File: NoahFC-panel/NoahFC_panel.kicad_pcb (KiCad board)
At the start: 2 copper layers, 97 x 97 mm, 112 parts, among them J1 CH1, J10 GND, J11 CH1, J12 CH2, J13 MPU6050, J14 FTDI, J15 8.4V, J16 CH3, J17 PPM, J18 GPS, J19 CH4, J2 CH2, J20 GND, J21 CH1, J22 CH2, J23 MPU6050, J24 FTDI, J25 8.4V, J26 CH3, J27 PPM, J28 GPS, J29 CH4, J3 MPU6050, J30 GND, J31 CH1, J32 CH2, J33 MPU6050, J34 FTDI, J35 8.4V, J36 CH3, J37 PPM, J38 GPS, J39 CH4, J4 FTDI, J40 GND, J5 8.4V, J6 CH3, J7 PPM, J8 GPS, J9 CH4, U1 ATmega328-A, U2 ATmega328-A, U3 AMS1117-5.0, U4 AMS1117-5.0, U5 ATmega328-A, U6 AMS1117-5.0, U7 ATmega328-A, U8 AMS1117-5.0, Y1 16Mhz, Y2 16Mhz, Y3 16Mhz, Y4 16Mhz

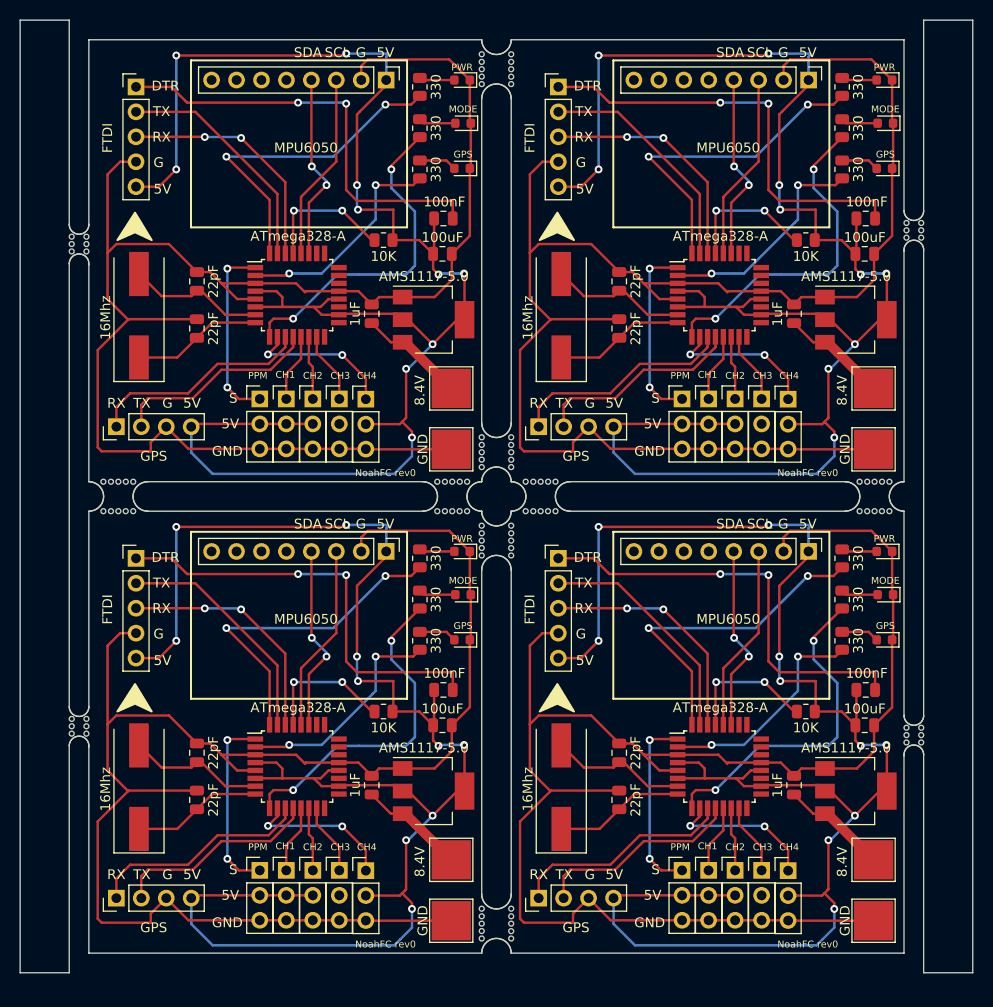
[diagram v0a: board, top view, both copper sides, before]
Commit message: fill board
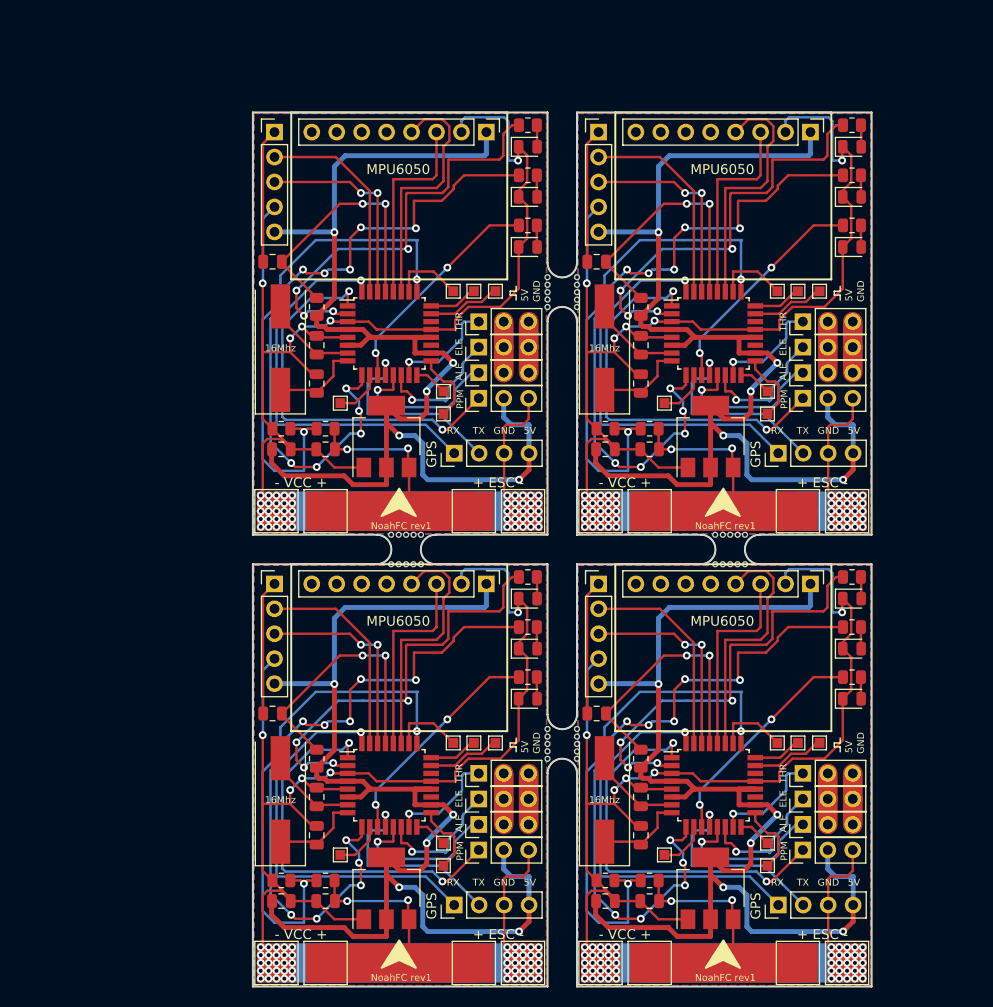
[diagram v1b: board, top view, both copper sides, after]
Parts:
- removed the C1 at (96.9, 72.9)
- removed C10, C15, C20: 100uF, Capacitor_SMD:C_0805_2012Metric
- removed C11, C12, C16, C17, C6, C7: 22pF, Capacitor_SMD:C_0805_2012Metric
- removed C13, C18, C8: 100nF, Capacitor_SMD:C_0805_2012Metric
- removed C14, C19, C9: 1uF, Capacitor_SMD:C_0805_2012Metric
- removed the C2 at (96.9, 77.7)
- removed the C3 at (122.0, 66.5)
- removed the C4 at (114.7, 76.2)
- removed the C5 at (121.9, 70.1)
- removed the D1 at (123.9, 52.4)
- removed D10, D4, D7: PWR, LED_SMD:LED_0603_1608Metric
- removed D11, D5, D8: GPS, LED_SMD:LED_0603_1608Metric
- removed D12, D6, D9: MODE, LED_SMD:LED_0603_1608Metric
- removed the D2 at (123.9, 61.4)
- removed the D3 at (124.0, 56.8)
- removed the J1 at (106.0, 84.9)
- removed the J10 at (122.8, 90.0)
- removed the J11 at (149.0, 84.9)
- removed the J12 at (151.7, 84.9)
- removed the J13 at (159.2, 52.4)
- removed the J14 at (133.7, 53.1)
- removed the J15 at (165.8, 83.8)
- removed the J16 at (154.4, 84.9)
- removed the J17 at (146.3, 84.9)
- removed J18, J28, J38: GPS, Connector_PinHeader_2.54mm:PinHeader_1x04_P2.54mm_Vertical
- removed J19, J29, J39: CH4, Connector_PinHeader_2.54mm:PinHeader_1x03_P2.54mm_Vertical
- removed the J2 at (108.7, 84.9)
- removed J20, J30, J40: GND, TestPoint:TestPoint_Pad_4.0x4.0mm
- removed J21, J31: CH1, Connector_PinHeader_2.54mm:PinHeader_1x03_P2.54mm_Vertical
- removed J22, J32: CH2, Connector_PinHeader_2.54mm:PinHeader_1x03_P2.54mm_Vertical
- removed J23, J33: MPU6050, Connector_PinHeader_2.54mm:PinHeader_1x08_P2.54mm_Vertical
- removed J24, J34: FTDI, Connector_PinHeader_2.54mm:PinHeader_1x05_P2.54mm_Vertical
- removed J25, J35: 8.4V, TestPoint:TestPoint_Pad_4.0x4.0mm
- removed J26, J36: CH3, Connector_PinHeader_2.54mm:PinHeader_1x03_P2.54mm_Vertical
- removed J27, J37: PPM, Connector_PinHeader_2.54mm:PinHeader_1x03_P2.54mm_Vertical
- removed the J3 at (116.2, 52.4)
- removed the J4 at (90.7, 53.1)
- removed the J5 at (122.8, 83.8)
- removed the J6 at (111.4, 84.9)
- removed the J7 at (103.3, 84.9)
- removed the J8 at (88.7, 87.7)
- removed the J9 at (114.1, 84.9)
- removed the R1 at (115.9, 68.7)
- removed R10, R11, R12, R14, R15, R16, R7, R8: 330, Resistor_SMD:R_0805_2012Metric
- removed R13, R9: 10K, Resistor_SMD:R_0805_2012Metric
- removed the R2 at (119.6, 53.1)
- removed the R3 at (119.6, 61.5)
- removed the R4 at (119.6, 57.3)
- removed the R5 at (158.9, 68.7)
- removed the R6 at (162.6, 53.1)
- removed the U1 at (107.1, 74.3)
- removed U2, U5, U7: ATmega328-A, Package_QFP:TQFP-32_7x7mm_P0.8mm
- removed the U3 at (121.0, 76.8)
- removed U4, U6, U8: AMS1117-5.0, Package_TO_SOT_SMD:SOT-223-3_TabPin2
- removed the Y1 at (91.0, 76.4)
- removed Y2, Y3, Y4: 16Mhz, Crystal:Crystal_SMD_HC49-SD
- removed the mouse-bite-3mm-slot at (84.9, 118.2)
- removed the mouse-bite-3mm-slot at (84.9, 69.1)
- removed the mouse-bite-3mm-slot at (131.9, 94.8)
- removed the mouse-bite-3mm-slot at (88.9, 94.8)
- removed the mouse-bite-3mm-slot at (169.9, 67.7)
- removed the mouse-bite-3mm-slot at (127.4, 51.3)
- removed the mouse-bite-3mm-slot at (127.4, 99.3)
- removed the mouse-bite-3mm-slot at (127.4, 90.3)
- removed the mouse-bite-3mm-slot at (127.4, 138.3)
- removed the mouse-bite-3mm-slot at (122.9, 94.8)
- removed the mouse-bite-3mm-slot at (169.9, 119.1)
- removed the mouse-bite-3mm-slot at (165.9, 94.8)
- added C1: 22pF, Capacitor_SMD:C_0805_2012Metric, F.Cu at (142.1, 125.4)
- added C1: 22pF, Capacitor_SMD:C_0805_2012Metric, F.Cu at (142.1, 79.4)
- added C1: 22pF, Capacitor_SMD:C_0805_2012Metric, F.Cu at (109.1, 125.4)
- added C1: 22pF, Capacitor_SMD:C_0805_2012Metric, F.Cu at (109.1, 79.4)
- added C2: 22pF, Capacitor_SMD:C_0805_2012Metric, F.Cu at (142.1, 129.3)
- added C2: 22pF, Capacitor_SMD:C_0805_2012Metric, F.Cu at (142.1, 83.3)
- added C2: 22pF, Capacitor_SMD:C_0805_2012Metric, F.Cu at (109.1, 83.3)
- added C2: 22pF, Capacitor_SMD:C_0805_2012Metric, F.Cu at (109.1, 129.3)
- added C3: 1nF, Capacitor_SMD:C_0805_2012Metric, F.Cu at (137.6, 70.9)
- added C3: 1nF, Capacitor_SMD:C_0805_2012Metric, F.Cu at (104.6, 70.9)
- added C3: 1nF, Capacitor_SMD:C_0805_2012Metric, F.Cu at (104.6, 116.9)
- added C3: 1nF, Capacitor_SMD:C_0805_2012Metric, F.Cu at (137.6, 116.9)
- added C4: 1uF, Capacitor_SMD:C_0805_2012Metric, F.Cu at (110.0, 136.0)
- added C4: 1uF, Capacitor_SMD:C_0805_2012Metric, F.Cu at (110.0, 90.0)
- added C4: 1uF, Capacitor_SMD:C_0805_2012Metric, F.Cu at (143.0, 90.0)
- added C4: 1uF, Capacitor_SMD:C_0805_2012Metric, F.Cu at (143.0, 136.0)
- added C5: 10uF, Capacitor_SMD:C_0805_2012Metric, F.Cu at (105.5, 136.0)
- added C5: 10uF, Capacitor_SMD:C_0805_2012Metric, F.Cu at (105.5, 90.0)
- added C5: 10uF, Capacitor_SMD:C_0805_2012Metric, F.Cu at (138.5, 90.0)
- added C5: 10uF, Capacitor_SMD:C_0805_2012Metric, F.Cu at (138.5, 136.0)
- added D1: GPS, LED_SMD:LED_0805_2012Metric, F.Cu at (130.6, 110.3)
- added D1: GPS, LED_SMD:LED_0805_2012Metric, F.Cu at (163.6, 110.3)
- added D1: GPS, LED_SMD:LED_0805_2012Metric, F.Cu at (130.6, 64.3)
- added D1: GPS, LED_SMD:LED_0805_2012Metric, F.Cu at (163.6, 64.3)
- added D2: MODE, LED_SMD:LED_0805_2012Metric, F.Cu at (130.6, 59.2)
- added D2: MODE, LED_SMD:LED_0805_2012Metric, F.Cu at (163.6, 59.2)
- added D2: MODE, LED_SMD:LED_0805_2012Metric, F.Cu at (163.6, 105.2)
- added D2: MODE, LED_SMD:LED_0805_2012Metric, F.Cu at (130.6, 105.2)
- added D3: PWR, LED_SMD:LED_0805_2012Metric, F.Cu at (163.6, 69.4)
- added D3: PWR, LED_SMD:LED_0805_2012Metric, F.Cu at (163.6, 115.4)
- added D3: PWR, LED_SMD:LED_0805_2012Metric, F.Cu at (130.6, 115.4)
- added D3: PWR, LED_SMD:LED_0805_2012Metric, F.Cu at (130.6, 69.4)
- added J1: ALE, Connector_PinHeader_2.54mm:PinHeader_1x03_P2.54mm_Vertical, F.Cu at (125.6, 128.2)
- added J1: ALE, Connector_PinHeader_2.54mm:PinHeader_1x03_P2.54mm_Vertical, F.Cu at (158.6, 128.2)
- added J1: ALE, Connector_PinHeader_2.54mm:PinHeader_1x03_P2.54mm_Vertical, F.Cu at (158.6, 82.2)
- added J1: ALE, Connector_PinHeader_2.54mm:PinHeader_1x03_P2.54mm_Vertical, F.Cu at (125.6, 82.2)
- added J10: GND, TestPoint:TestPoint_Pad_4.0x4.0mm, F.Cu at (105.0, 142.3)
- added J10: GND, TestPoint:TestPoint_Pad_4.0x4.0mm, F.Cu at (138.0, 142.3)
- added J10: GND, TestPoint:TestPoint_Pad_4.0x4.0mm, F.Cu at (138.0, 96.3)
- added J10: GND, TestPoint:TestPoint_Pad_4.0x4.0mm, F.Cu at (105.0, 96.3)
- added J11: SCK, TestPoint:TestPoint_Pad_1.0x1.0mm, F.Cu at (155.0, 132.4)
- added J11: SCK, TestPoint:TestPoint_Pad_1.0x1.0mm, F.Cu at (155.0, 86.4)
- added J11: SCK, TestPoint:TestPoint_Pad_1.0x1.0mm, F.Cu at (122.0, 132.4)
- added J11: SCK, TestPoint:TestPoint_Pad_1.0x1.0mm, F.Cu at (122.0, 86.4)
- added J12: MISO, TestPoint:TestPoint_Pad_1.0x1.0mm, F.Cu at (155.0, 130.1)
- added J12: MISO, TestPoint:TestPoint_Pad_1.0x1.0mm, F.Cu at (155.0, 84.1)
- added J12: MISO, TestPoint:TestPoint_Pad_1.0x1.0mm, F.Cu at (122.0, 130.1)
- added J12: MISO, TestPoint:TestPoint_Pad_1.0x1.0mm, F.Cu at (122.0, 84.1)
- added J13: VCC, TestPoint:TestPoint_Pad_4.0x4.0mm, F.Cu at (158.1, 142.3)
- added J13: VCC, TestPoint:TestPoint_Pad_4.0x4.0mm, F.Cu at (158.1, 96.3)
- added J13: VCC, TestPoint:TestPoint_Pad_4.0x4.0mm, F.Cu at (125.1, 142.3)
- added J13: VCC, TestPoint:TestPoint_Pad_4.0x4.0mm, F.Cu at (125.1, 96.3)
- added J14: GND, TestPoint:TestPoint_Pad_4.0x4.0mm, F.Cu at (130.1, 142.3)
- added J14: GND, TestPoint:TestPoint_Pad_4.0x4.0mm, F.Cu at (163.1, 142.3)
- added J14: GND, TestPoint:TestPoint_Pad_4.0x4.0mm, F.Cu at (130.1, 96.3)
- added J14: GND, TestPoint:TestPoint_Pad_4.0x4.0mm, F.Cu at (163.1, 96.3)
- added J15: A1, TestPoint:TestPoint_Pad_1.0x1.0mm, F.Cu at (125.1, 73.9)
- added J15: A1, TestPoint:TestPoint_Pad_1.0x1.0mm, F.Cu at (158.1, 119.9)
- added J15: A1, TestPoint:TestPoint_Pad_1.0x1.0mm, F.Cu at (125.1, 119.9)
- added J15: A1, TestPoint:TestPoint_Pad_1.0x1.0mm, F.Cu at (158.1, 73.9)
- added J16: A3, TestPoint:TestPoint_Pad_1.0x1.0mm, F.Cu at (156.0, 73.9)
- added J16: A3, TestPoint:TestPoint_Pad_1.0x1.0mm, F.Cu at (123.0, 119.9)
- added J16: A3, TestPoint:TestPoint_Pad_1.0x1.0mm, F.Cu at (156.0, 119.9)
- added J16: A3, TestPoint:TestPoint_Pad_1.0x1.0mm, F.Cu at (123.0, 73.9)
- added J17: D6, TestPoint:TestPoint_Pad_1.0x1.0mm, F.Cu at (111.5, 85.3)
- added J17: D6, TestPoint:TestPoint_Pad_1.0x1.0mm, F.Cu at (144.5, 131.3)
- added J17: D6, TestPoint:TestPoint_Pad_1.0x1.0mm, F.Cu at (144.5, 85.3)
- added J17: D6, TestPoint:TestPoint_Pad_1.0x1.0mm, F.Cu at (111.5, 131.3)
- added J2: ELE, Connector_PinHeader_2.54mm:PinHeader_1x03_P2.54mm_Vertical, F.Cu at (125.6, 79.6)
- added J2: ELE, Connector_PinHeader_2.54mm:PinHeader_1x03_P2.54mm_Vertical, F.Cu at (158.6, 79.6)
- added J2: ELE, Connector_PinHeader_2.54mm:PinHeader_1x03_P2.54mm_Vertical, F.Cu at (158.6, 125.6)
- added J2: ELE, Connector_PinHeader_2.54mm:PinHeader_1x03_P2.54mm_Vertical, F.Cu at (125.6, 125.6)
- added J3: MPU6050, Connector_PinHeader_2.54mm:PinHeader_1x08_P2.54mm_Vertical, F.Cu at (126.4, 103.7)
- added J3: MPU6050, Connector_PinHeader_2.54mm:PinHeader_1x08_P2.54mm_Vertical, F.Cu at (126.4, 57.7)
- added J3: MPU6050, Connector_PinHeader_2.54mm:PinHeader_1x08_P2.54mm_Vertical, F.Cu at (159.4, 57.7)
- added J3: MPU6050, Connector_PinHeader_2.54mm:PinHeader_1x08_P2.54mm_Vertical, F.Cu at (159.4, 103.7)
- added J4: FTDI, Connector_PinHeader_2.54mm:PinHeader_1x05_P2.54mm_Vertical, F.Cu at (137.8, 103.7)
- added J4: FTDI, Connector_PinHeader_2.54mm:PinHeader_1x05_P2.54mm_Vertical, F.Cu at (104.8, 57.7)
- added J4: FTDI, Connector_PinHeader_2.54mm:PinHeader_1x05_P2.54mm_Vertical, F.Cu at (104.8, 103.7)
- added J4: FTDI, Connector_PinHeader_2.54mm:PinHeader_1x05_P2.54mm_Vertical, F.Cu at (137.8, 57.7)
- added J5: VCC, TestPoint:TestPoint_Pad_4.0x4.0mm, F.Cu at (143.0, 96.3)
- added J5: VCC, TestPoint:TestPoint_Pad_4.0x4.0mm, F.Cu at (110.0, 142.3)
- added J5: VCC, TestPoint:TestPoint_Pad_4.0x4.0mm, F.Cu at (143.0, 142.3)
- added J5: VCC, TestPoint:TestPoint_Pad_4.0x4.0mm, F.Cu at (110.0, 96.3)
- added J6: THR, Connector_PinHeader_2.54mm:PinHeader_1x03_P2.54mm_Vertical, F.Cu at (125.6, 77.0)
- added J6: THR, Connector_PinHeader_2.54mm:PinHeader_1x03_P2.54mm_Vertical, F.Cu at (158.6, 77.0)
- added J6: THR, Connector_PinHeader_2.54mm:PinHeader_1x03_P2.54mm_Vertical, F.Cu at (125.6, 123.0)
- added J6: THR, Connector_PinHeader_2.54mm:PinHeader_1x03_P2.54mm_Vertical, F.Cu at (158.6, 123.0)
- added J7: PPM, Connector_PinHeader_2.54mm:PinHeader_1x03_P2.54mm_Vertical, F.Cu at (125.6, 84.8)
- added J7: PPM, Connector_PinHeader_2.54mm:PinHeader_1x03_P2.54mm_Vertical, F.Cu at (158.6, 130.8)
- added J7: PPM, Connector_PinHeader_2.54mm:PinHeader_1x03_P2.54mm_Vertical, F.Cu at (125.6, 130.8)
- added J7: PPM, Connector_PinHeader_2.54mm:PinHeader_1x03_P2.54mm_Vertical, F.Cu at (158.6, 84.8)
- added J8: GPS, Connector_PinHeader_2.54mm:PinHeader_1x04_P2.54mm_Vertical, F.Cu at (156.1, 136.4)
- added J8: GPS, Connector_PinHeader_2.54mm:PinHeader_1x04_P2.54mm_Vertical, F.Cu at (123.1, 136.4)
- added J8: GPS, Connector_PinHeader_2.54mm:PinHeader_1x04_P2.54mm_Vertical, F.Cu at (123.1, 90.4)
- added J8: GPS, Connector_PinHeader_2.54mm:PinHeader_1x04_P2.54mm_Vertical, F.Cu at (156.1, 90.4)
- added J9: A0, TestPoint:TestPoint_Pad_1.0x1.0mm, F.Cu at (160.3, 73.9)
- added J9: A0, TestPoint:TestPoint_Pad_1.0x1.0mm, F.Cu at (127.3, 119.9)
- added J9: A0, TestPoint:TestPoint_Pad_1.0x1.0mm, F.Cu at (127.3, 73.9)
- added J9: A0, TestPoint:TestPoint_Pad_1.0x1.0mm, F.Cu at (160.3, 119.9)
- added R1: 10K, Resistor_SMD:R_0805_2012Metric, F.Cu at (142.1, 75.5)
- added R1: 10K, Resistor_SMD:R_0805_2012Metric, F.Cu at (109.1, 75.5)
- added R1: 10K, Resistor_SMD:R_0805_2012Metric, F.Cu at (109.1, 121.5)
- added R1: 10K, Resistor_SMD:R_0805_2012Metric, F.Cu at (142.1, 121.5)
- added R2: 330, Resistor_SMD:R_0805_2012Metric, F.Cu at (130.6, 108.1)
- added R2: 330, Resistor_SMD:R_0805_2012Metric, F.Cu at (163.6, 108.1)
- added R2: 330, Resistor_SMD:R_0805_2012Metric, F.Cu at (130.6, 62.1)
- added R2: 330, Resistor_SMD:R_0805_2012Metric, F.Cu at (163.6, 62.1)
- added R3: 330, Resistor_SMD:R_0805_2012Metric, F.Cu at (163.6, 57.0)
- added R3: 330, Resistor_SMD:R_0805_2012Metric, F.Cu at (130.6, 103.0)
- added R3: 330, Resistor_SMD:R_0805_2012Metric, F.Cu at (130.6, 57.0)
- added R3: 330, Resistor_SMD:R_0805_2012Metric, F.Cu at (163.6, 103.0)
- added R4: 330, Resistor_SMD:R_0805_2012Metric, F.Cu at (163.6, 113.2)
- added R4: 330, Resistor_SMD:R_0805_2012Metric, F.Cu at (130.6, 67.2)
- added R4: 330, Resistor_SMD:R_0805_2012Metric, F.Cu at (163.6, 67.2)
- added R4: 330, Resistor_SMD:R_0805_2012Metric, F.Cu at (130.6, 113.2)
- added R5: 100K, Resistor_SMD:R_0805_2012Metric, F.Cu at (143.0, 133.9)
- added R5: 100K, Resistor_SMD:R_0805_2012Metric, F.Cu at (110.0, 87.9)
- added R5: 100K, Resistor_SMD:R_0805_2012Metric, F.Cu at (110.0, 133.9)
- added R5: 100K, Resistor_SMD:R_0805_2012Metric, F.Cu at (143.0, 87.9)
- added R6: 10K, Resistor_SMD:R_0805_2012Metric, F.Cu at (105.5, 87.9)
- added R6: 10K, Resistor_SMD:R_0805_2012Metric, F.Cu at (138.5, 87.9)
- added R6: 10K, Resistor_SMD:R_0805_2012Metric, F.Cu at (105.5, 133.9)
- added R6: 10K, Resistor_SMD:R_0805_2012Metric, F.Cu at (138.5, 133.9)
- added U1: ATmega328, Package_QFP:TQFP-32_7x7mm_P0.8mm, F.Cu at (116.5, 124.2)
- added U1: ATmega328, Package_QFP:TQFP-32_7x7mm_P0.8mm, F.Cu at (149.5, 78.2)
- added U1: ATmega328, Package_QFP:TQFP-32_7x7mm_P0.8mm, F.Cu at (116.5, 78.2)
- added U1: ATmega328, Package_QFP:TQFP-32_7x7mm_P0.8mm, F.Cu at (149.5, 124.2)
- added U3: AMS1117-5.0, Package_TO_SOT_SMD:SOT-223-3_TabPin2, F.Cu at (116.2, 88.7)
- added U3: AMS1117-5.0, Package_TO_SOT_SMD:SOT-223-3_TabPin2, F.Cu at (149.2, 88.7)
- added U3: AMS1117-5.0, Package_TO_SOT_SMD:SOT-223-3_TabPin2, F.Cu at (149.2, 134.7)
- added U3: AMS1117-5.0, Package_TO_SOT_SMD:SOT-223-3_TabPin2, F.Cu at (116.2, 134.7)
- added Y1: 16Mhz, Crystal:Crystal_SMD_HC49-SD, F.Cu at (138.4, 125.7)
- added Y1: 16Mhz, Crystal:Crystal_SMD_HC49-SD, F.Cu at (105.4, 125.7)
- added Y1: 16Mhz, Crystal:Crystal_SMD_HC49-SD, F.Cu at (138.4, 79.7)
- added Y1: 16Mhz, Crystal:Crystal_SMD_HC49-SD, F.Cu at (105.4, 79.7)
- added mouse-bite-3mm-slot: VAL**, TestPoint:mouse-bite-3mm-slot, F.Cu at (134.1, 74.0)
- added mouse-bite-3mm-slot: VAL**, TestPoint:mouse-bite-3mm-slot, F.Cu at (118.2, 100.2)
- added mouse-bite-3mm-slot1: VAL**, TestPoint:mouse-bite-3mm-slot, F.Cu at (151.2, 100.2)
- added mouse-bite-3mm-slot4: VAL**, TestPoint:mouse-bite-3mm-slot, F.Cu at (134.1, 120.0)
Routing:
- net (no net): track 2826.6 -> 3370.3 mm, vias 112 -> 364
- added copper zone on B.Cu, net (none)
- added copper zone on F.Cu, net (none)
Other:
- board size 97 x 97 mm -> 63 x 89 mm
- board text added: "+ ESC -"
- board text added: "- VCC +"
- board text added: "NoahFC rev1"
- board text added: "http://github.com/zosko/NoahFC by Bosko"
- board text removed: "G"
- board text removed: "NoahFC rev0"
- board text removed: "S"
